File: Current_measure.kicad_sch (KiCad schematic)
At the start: 12 parts

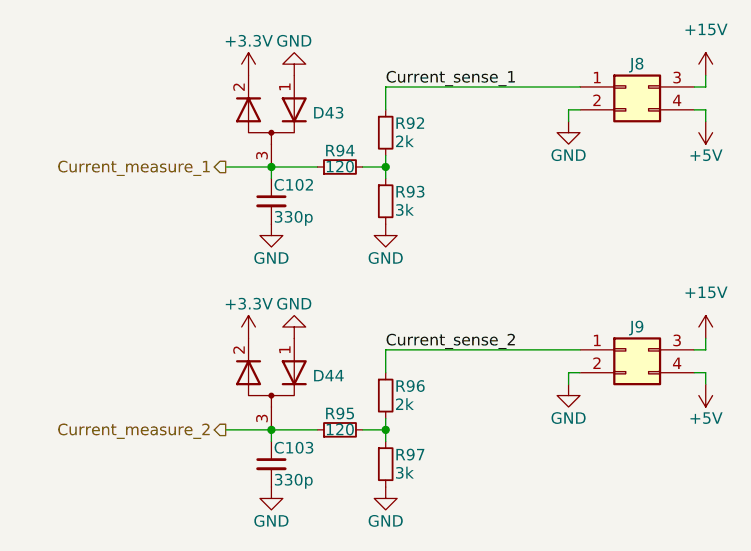
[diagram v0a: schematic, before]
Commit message: VER1.0: добавил разъемы для платы вторички
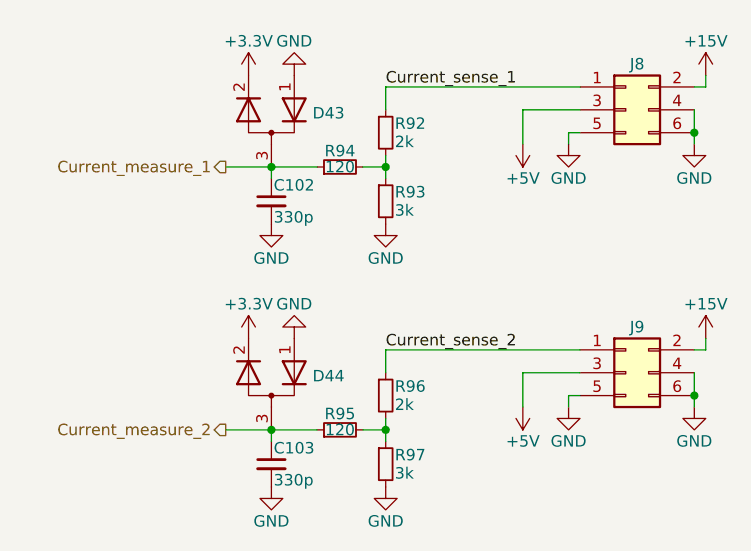
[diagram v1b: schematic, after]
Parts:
- removed J8, J9: (no value), symbol Connector_Generic:Conn_02x02_Top_Bottom
- added J8, J9: (no value), Connector_Molex:Molex_Mini-Fit_Jr_5569-06A2_2x03_P4.20mm_Horizontal, symbol Connector_Generic:Conn_02x03_Odd_Even
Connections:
- net +15V: now also J8.2 (Pin_2), J9.2 (Pin_2)
- net +5V: now also J8.3 (Pin_3), J9.3 (Pin_3)
- net Current_sense_1: now also J8.1 (Pin_1)
- net Current_sense_2: now also J9.1 (Pin_1)
- net GND: now also J8.4 (Pin_4), J8.5 (Pin_5), J8.6 (Pin_6), J9.4 (Pin_4), J9.5 (Pin_5), J9.6 (Pin_6)
